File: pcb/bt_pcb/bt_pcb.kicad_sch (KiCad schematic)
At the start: 0 parts

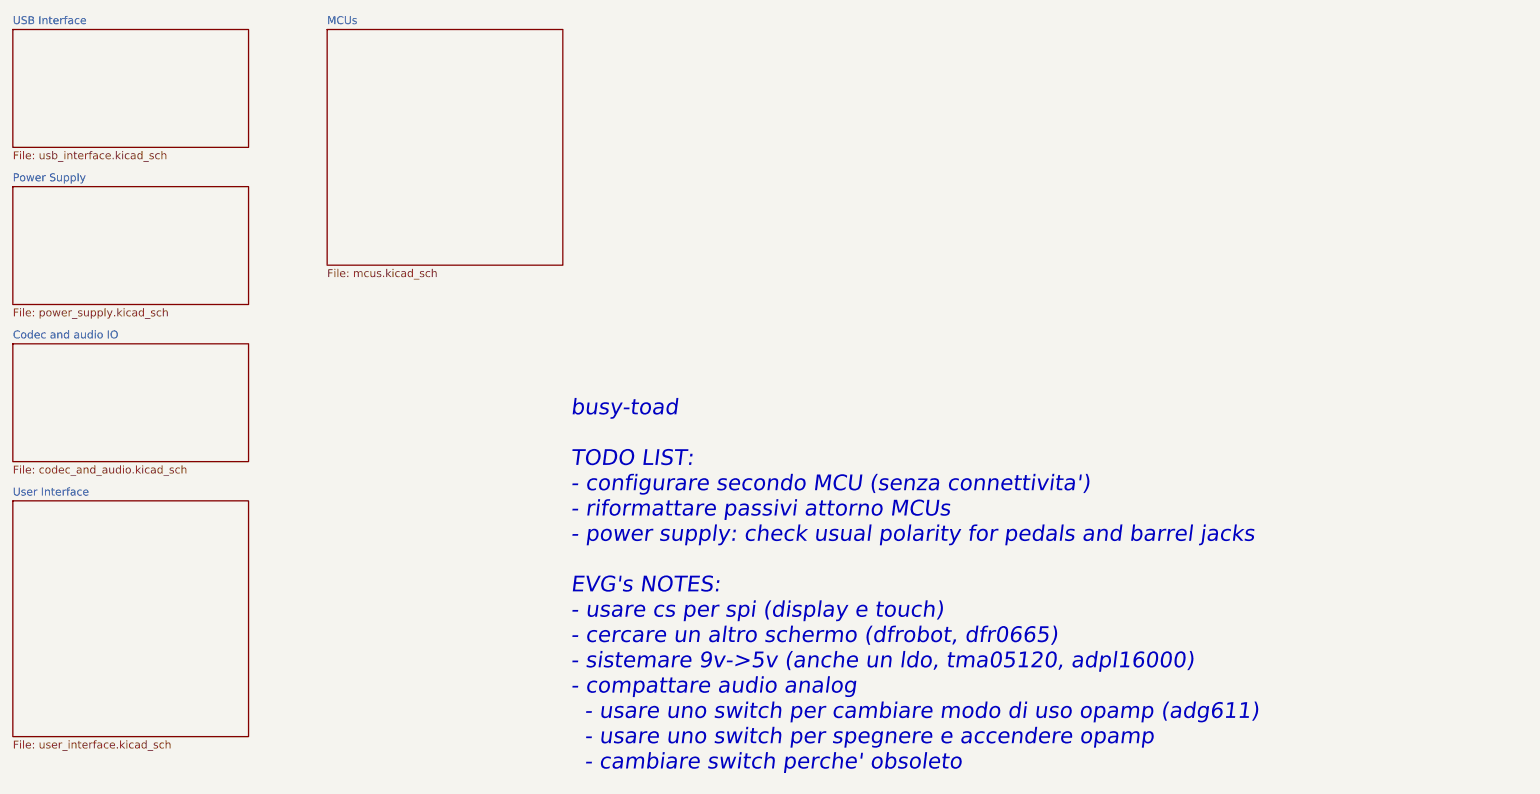
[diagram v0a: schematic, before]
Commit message: solving some erc warnings and errors
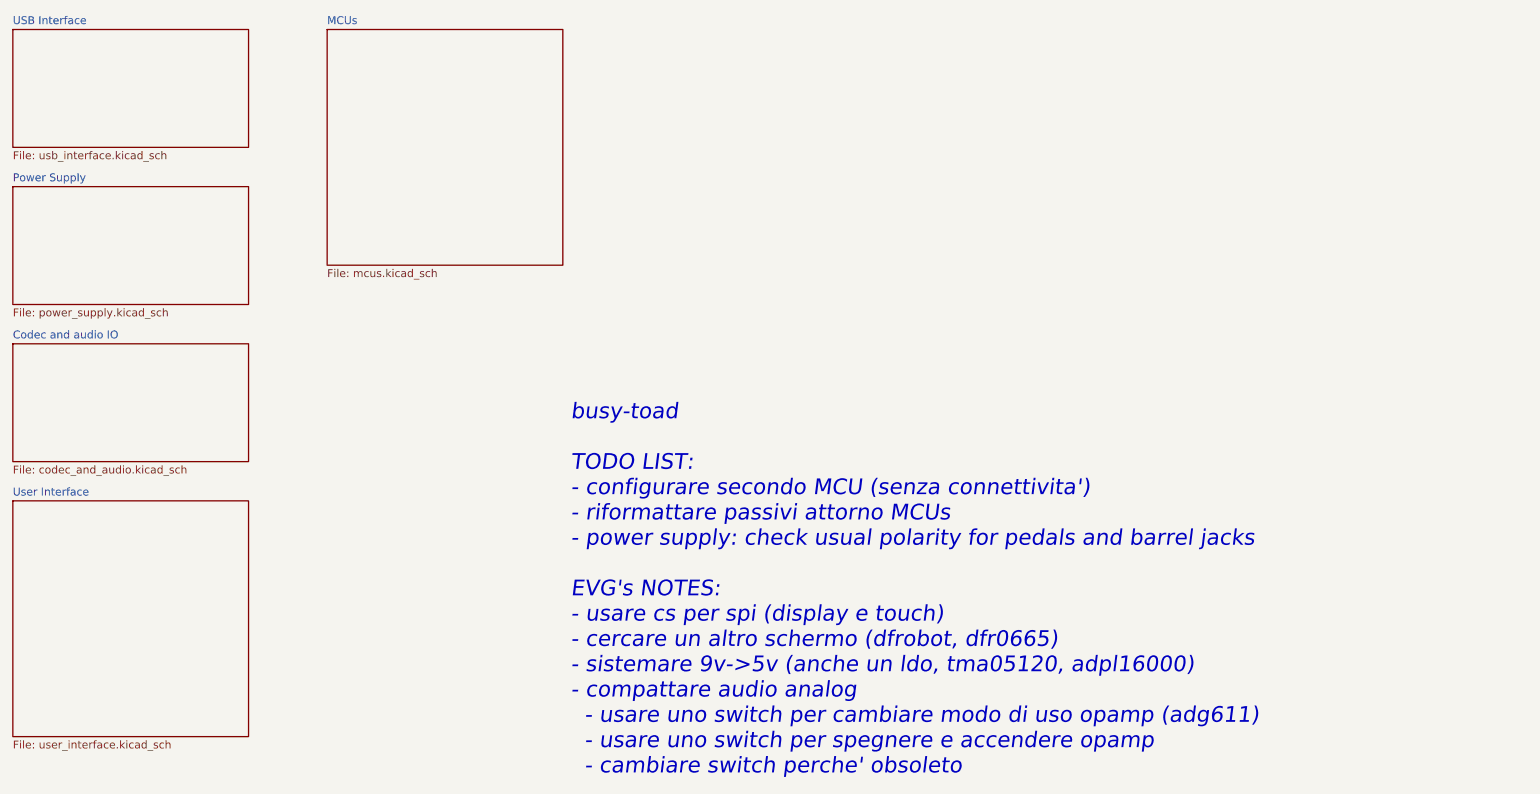
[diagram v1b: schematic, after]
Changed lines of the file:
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@@
 	(text "busy-toad\n\nTODO LIST:\n- configurare secondo MCU (senza connettivita')\n- riformattare passivi attorno MCUs\n- power supply: check usual polarity for pedals and barrel jacks\n\nEVG's NOTES:\n- usare cs per spi (display e touch)\n- cercare un altro schermo (dfrobot, dfr0665)\n- sistemare 9v->5v (anche un ldo, tma05120, adpl16000)\n- compattare audio analog\n  - usare uno switch per cambiare modo di uso opamp (adg611) \n  - usare uno switch per spegnere e accendere opamp\n  - cambiare switch perche' obsoleto\n"
 		(exclude_from_sim no)
-		(at 115.57 145.415 0)
+		(at 115.57 146.05 0)
 		(effects
 			(font
